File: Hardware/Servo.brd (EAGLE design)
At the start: 50 x 33 mm, 15 parts, among them T1 BC337, T2 BC337, U1 PIC16F1508-I/P

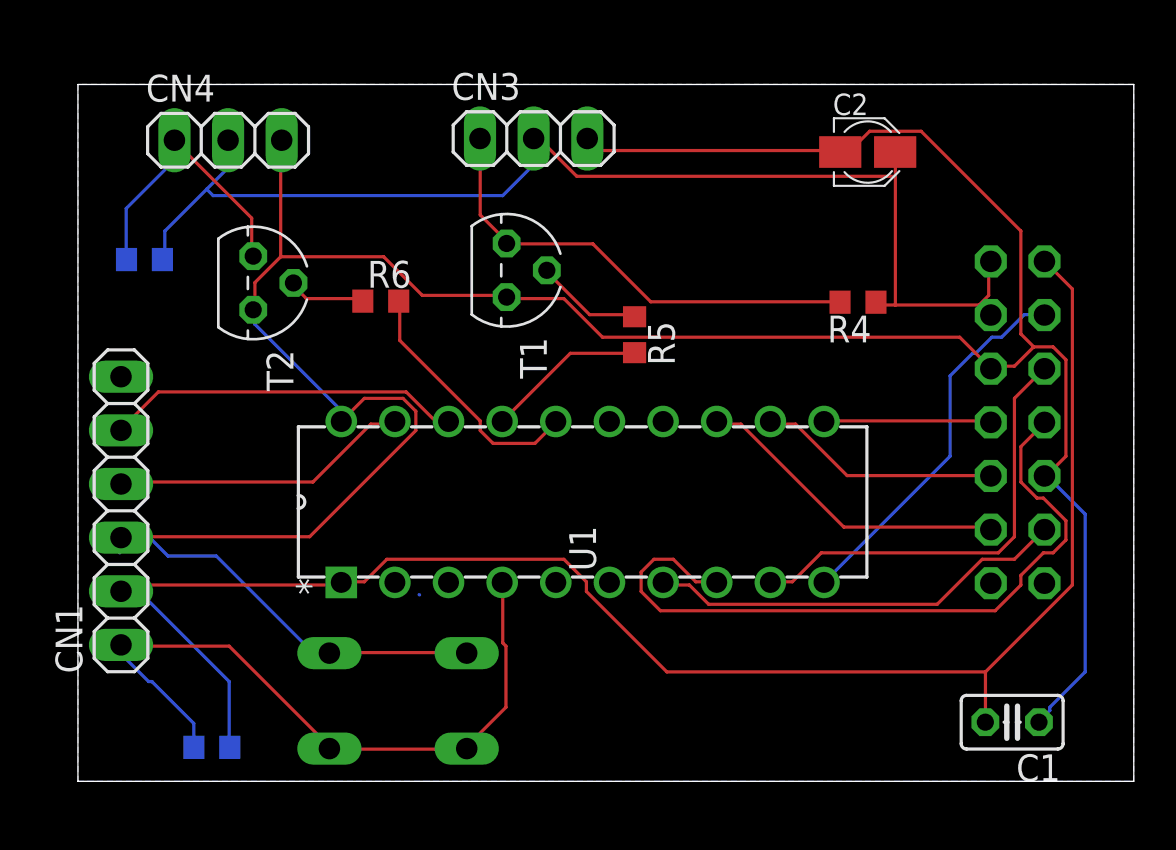
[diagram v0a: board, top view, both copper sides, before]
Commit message: 1/12
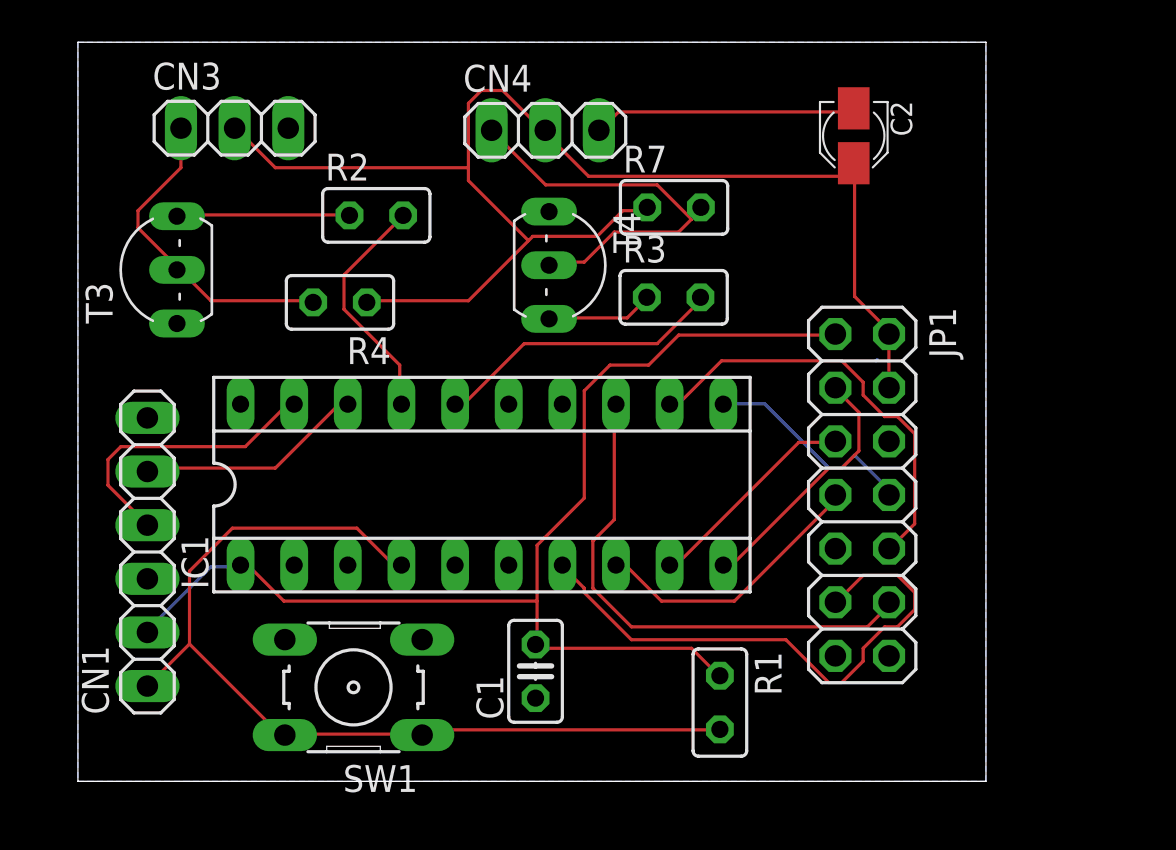
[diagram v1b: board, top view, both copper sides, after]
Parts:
- removed R5, R6: (no value), rcl:R0603
- removed T1, T2: BC337, transistor:TO92
- removed U1: PIC16F1508-I/P, pic16f1508:PDIP20_300MC
- added IC1: PIC16F1508, ic-package:SOCKET-20
- added R2, R3: 3.3k, rcl:V526-0
- added T3, T4: 2SC1815, transistor:TO92-ECB
- C1: value (none) -> 4.7uF
- C2: value (none) -> 100uF
- CN1: value (none) -> ICSP
- CN3: value (none) -> Servo1
- CN4: value (none) -> Servo2
- JP1: value (none) -> Raspi
- R1: value (none) -> 10k; device rcl:R0603 -> rcl:V526-0
- R4, R7: value (none) -> 5.1k; device rcl:R0603 -> rcl:V526-0
- SW1: value (none) -> Reset
- moved R7 25.2 mm to (28.2, 27.2), flipped to the top
- moved R4 24.5 mm to (12.4, 22.7)
- moved R1 24.2 mm to (30.4, 3.73), flipped to the top, turned to 270 degrees
- moved C1 22.7 mm to (21.7, 5.21), turned to 90 degrees
- moved CN4 15.0 mm to (22.1, 30.8)
- moved CN3 14.2 mm to (7.42, 30.9)
- moved JP1 8.12 mm to (37.1, 13.6), flipped to the top
- moved CN1 2.32 mm to (3.29, 10.9)
- moved SW1 2.20 mm to (13.1, 4.45), flipped to the top
- moved C2 1.01 mm to (36.7, 30.6), turned to 270 degrees
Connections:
- removed net N$10: JP1.10, U1.12
- removed net N$16: R6.2, U1.16
- removed net N$17: R5.1, T1.2
- removed net N$18: R6.1, T2.2
- removed net N$24: CN3.1, R4.2, T1.3
- new net N$12: IC1.16, R3.2
- new net N$13: R2.1, T3.B
- new net N$14: R3.1, T4.B
- new net N$6: IC1.11, JP1.8
- new net N$7: IC1.12, JP1.10
- net GND1: now also IC1.20, T3.E, T4.E; no longer T1.1, T2.1, U1.20
- net N$1: now also IC1.10; no longer U1.10
- net N$11: now also IC1.17, R2.2; no longer JP1.12, U1.13
- net N$15: now also CN3.1, R4.2, T3.C; no longer R5.2, U1.17
- net N$19: now also CN1.4, IC1.19; no longer CN1.5, U1.18
- net N$2: now also IC1.9; no longer U1.9
- net N$20: now also CN1.5, IC1.18; no longer CN1.4, U1.19
- net N$3: now also IC1.8; no longer U1.8
- net N$4: now also T4.C; no longer T2.3
- net N$5: now also IC1.7; no longer U1.7
- net N$8: now also IC1.4; no longer U1.4
- net N$9: now also IC1.13, JP1.12; no longer JP1.8, U1.11
- net VDD: now also IC1.1; no longer U1.1
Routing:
- net GND1: track 144.0 -> 12.5 mm
- net N$24: track 22.4 -> 0.00 mm
- net VDD: track 78.1 -> 55.9 mm
- net N$3: track 34.4 -> 13.4 mm
- net N$7: track 0.00 -> 20.2 mm
- net N$9: track 7.93 -> 24.5 mm
- net N$12: track 0.00 -> 13.8 mm
- net N$16: track 12.0 -> 0.00 mm
- net N$8: track 33.5 -> 45.1 mm
- net N$10: track 11.5 -> 0.09 mm
- net N$2: track 21.0 -> 10.3 mm
- net N$6: track 0.03 -> 10.5 mm
- net VCC: track 58.3 -> 66.9 mm
- net N$13: track 0.00 -> 8.18 mm
- net N$15: track 7.61 -> 15.4 mm
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- added copper zone on layer 16, net GND1
- removed copper zone on layer 16, net N$12
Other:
- board size 50 x 33 mm -> 43 x 35 mm
